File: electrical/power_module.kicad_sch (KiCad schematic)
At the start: 15 parts, among them J1 Screw_Terminal_01x01, J2 Screw_Terminal_01x01, J3 Ground connector from bulb wi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, Q1 IRF5305, Q2 BC547

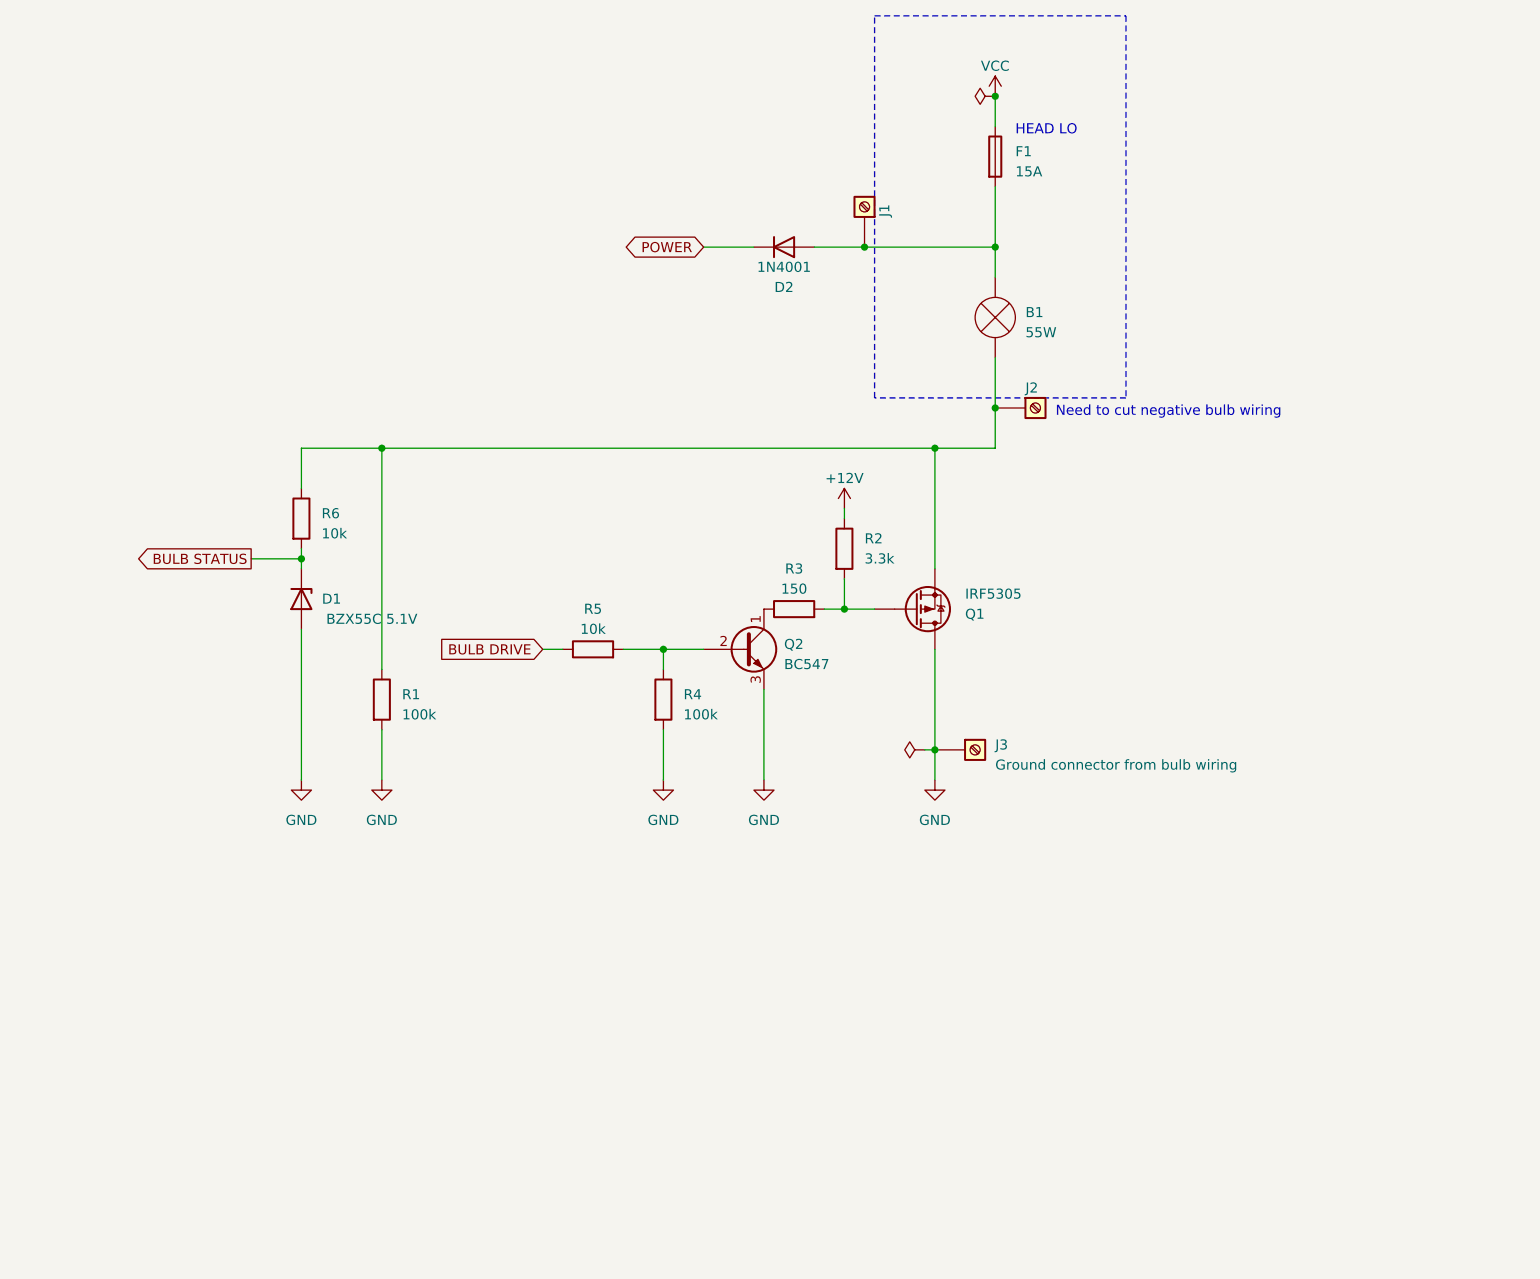
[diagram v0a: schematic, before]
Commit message: Fixes in power module
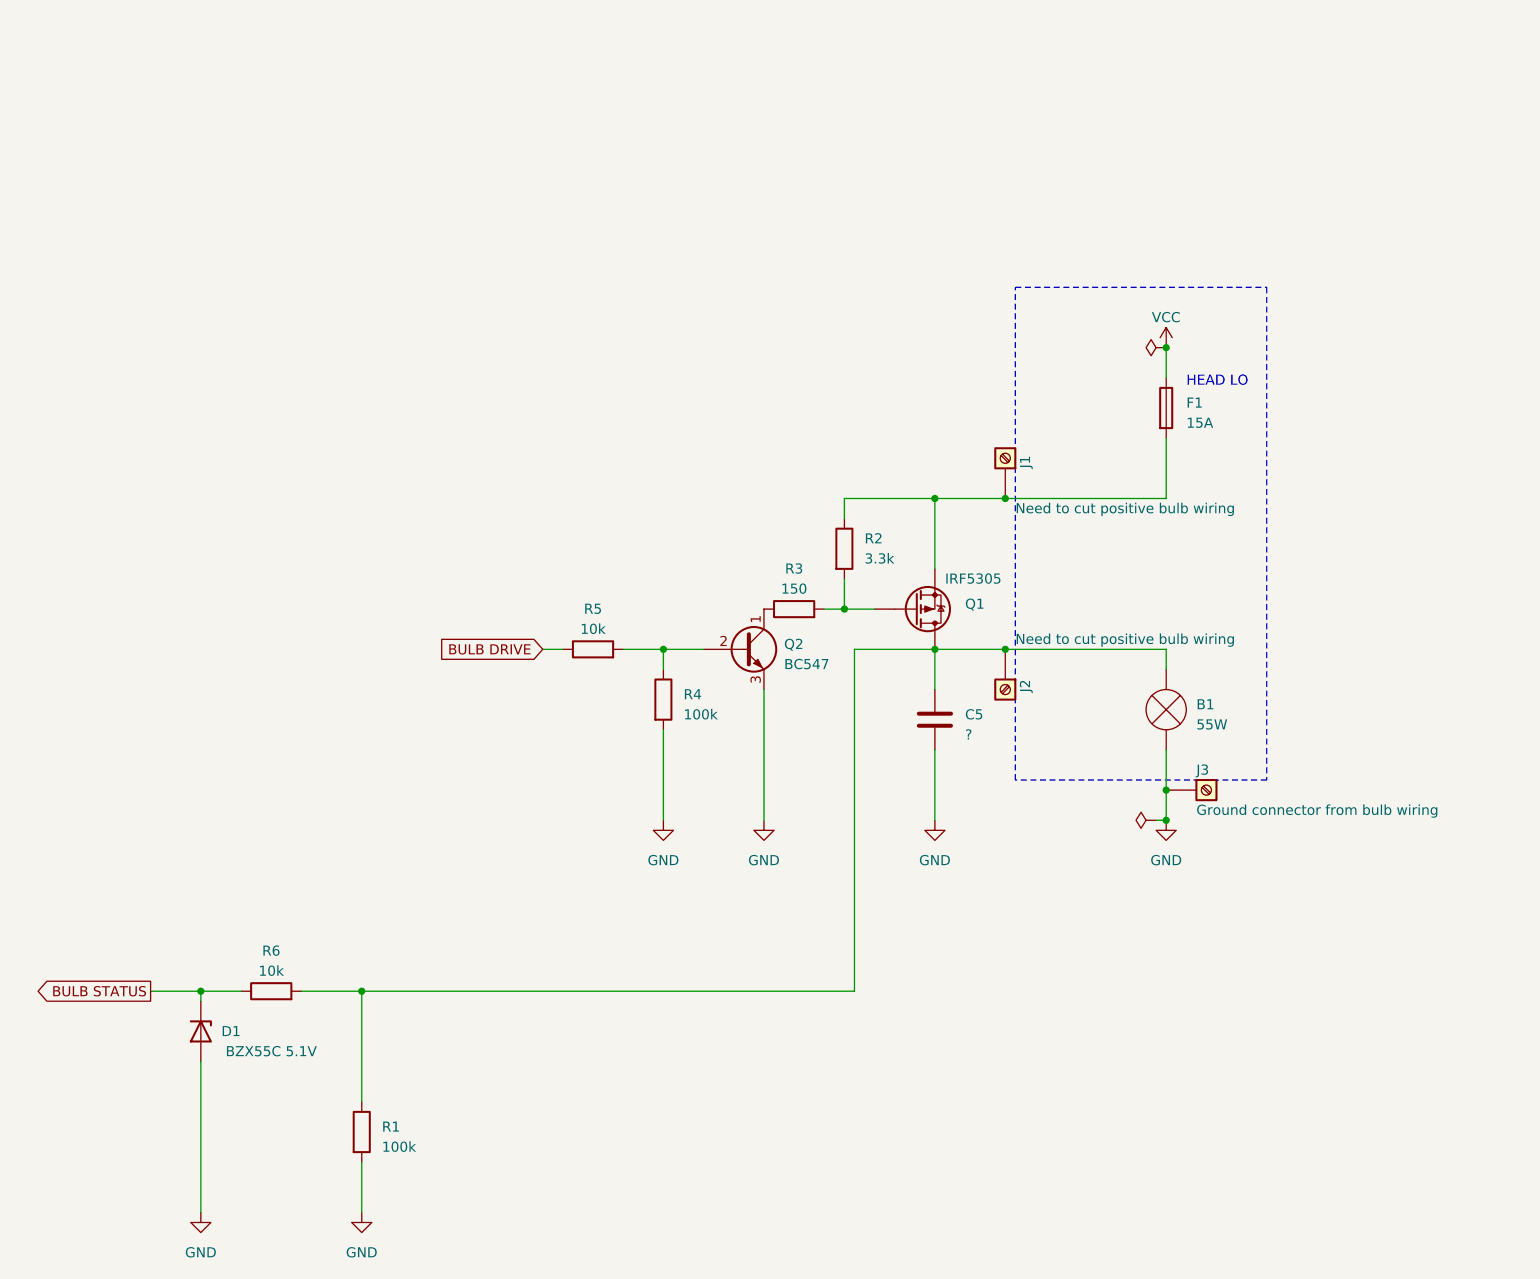
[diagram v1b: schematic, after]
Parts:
- removed D2: 1N4001, Diode_THT:D_DO-41_SOD81_P10.16mm_Horizontal, symbol Diode:1N4001
- added C5: ?, symbol Device:C
- J1, J2: value Screw_Terminal_01x01 -> Need to cut positive bulb wiring
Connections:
- net VDC is gone; now on an unnamed net: R2.1
- net BULB STATUS: now also R6.1; no longer R6.2
- net GND: now also B1.1 (-), C5.2; no longer Q1.2 (D)
- net at F1.2, J1.1 (Pin_1): now also Q1.3 (S); no longer B1.2 (+)
- new net: B1.2 (+), C5.1, J2.1 (Pin_1), Q1.2 (D), R1.1, R6.2
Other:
- note removed: "Need to cut negative bulb wiring"
- moved on the sheet: B1, D1, F1, J1, J2, J3, R1, R6
